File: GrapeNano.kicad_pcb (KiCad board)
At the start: 2 copper layers, 18.5 x 43.7 mm, 31 parts, among them P1 USB_OTG, P2 ICSP, SW1 SW_Push, U1 LM1117-5.0, U2 CH340G, U3 ATMEGA328P-AU, Y1 12MHz, Y2 16Mhz

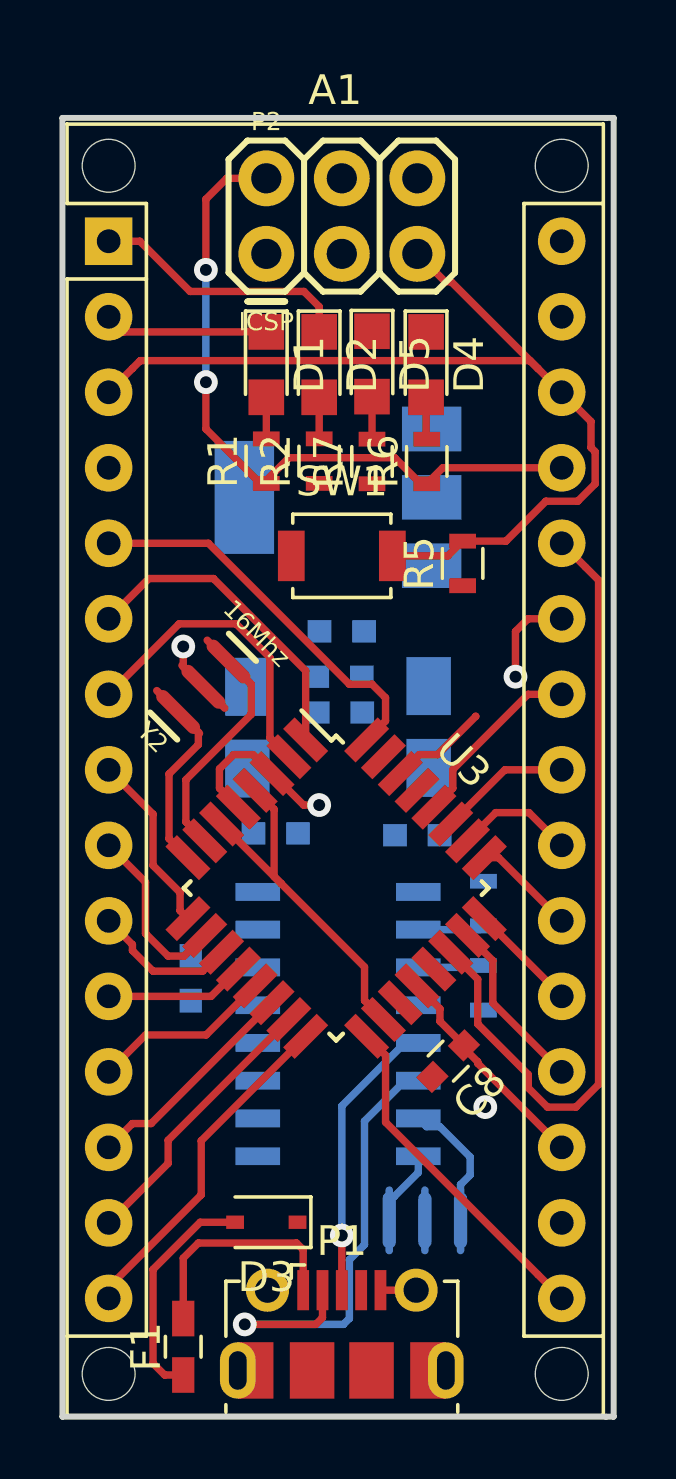
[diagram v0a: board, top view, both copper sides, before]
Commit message: 4 nets
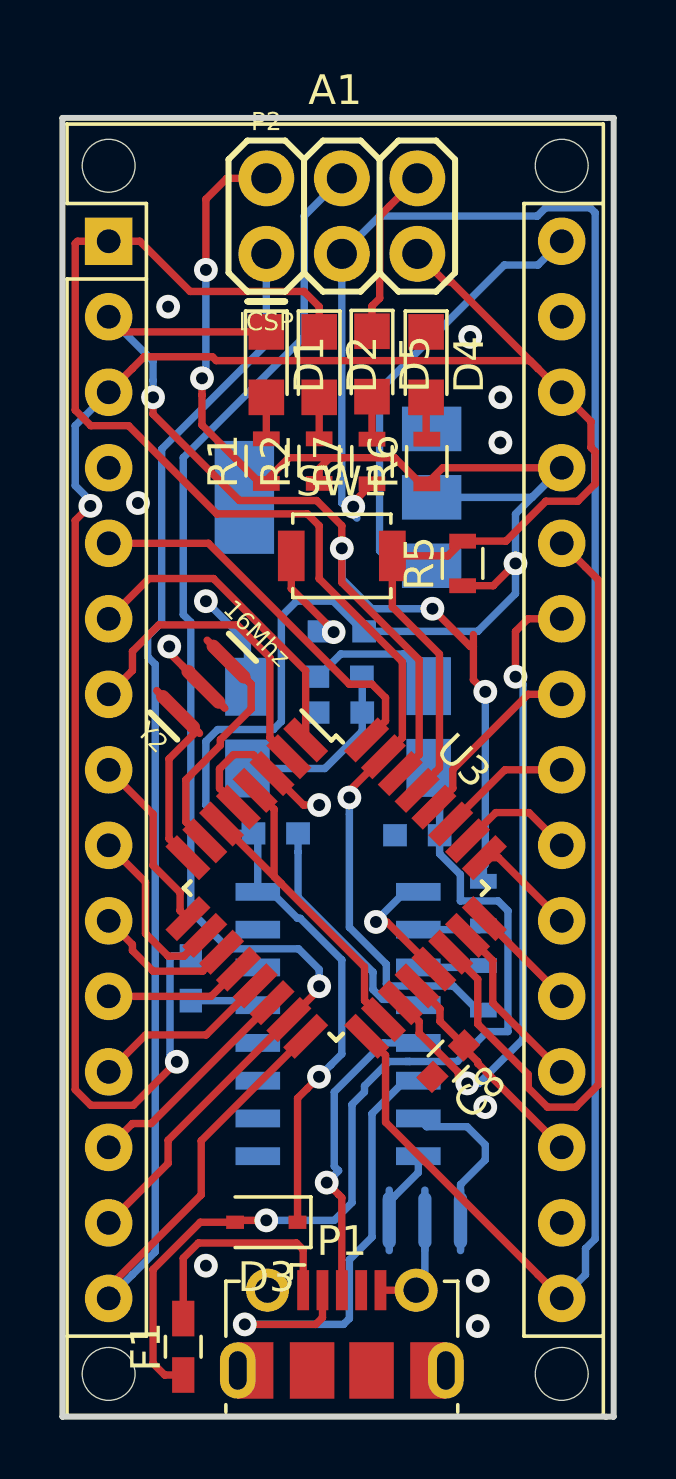
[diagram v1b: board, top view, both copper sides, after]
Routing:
- net D13-SCK: track 11.5 -> 68.0 mm, vias 0 -> 1
- net +5V: track 23.6 -> 71.6 mm, vias 2 -> 4
- net RESET: track 33.2 -> 75.1 mm, vias 0 -> 2
- net D1-TX: track 8.84 -> 46.9 mm, vias 0 -> 1
- net D12-MISO: track 11.6 -> 49.1 mm
- net D11-MOSI: track 9.35 -> 43.6 mm, vias 0 -> 1
- net D0-RX: track 8.86 -> 41.9 mm, vias 0 -> 4
- net VUSB: track 7.76 -> 32.5 mm, vias 0 -> 1
- net GND: track 8.64 -> 33.3 mm, vias 3 -> 12
- net A6: track 3.25 -> 21.8 mm, vias 1 -> 2
- net VIN: track 0.00 -> 15.6 mm
- net Net-(C1-Pad2): track 0.00 -> 8.04 mm
- net Net-(C6-Pad1): track 12.3 -> 18.6 mm
- net DTR: track 0.00 -> 2.32 mm
- net Net-(P1-Pad3): track 9.65 -> 10.6 mm
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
